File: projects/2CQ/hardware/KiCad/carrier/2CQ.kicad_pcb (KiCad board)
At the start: 2 copper layers, 48.5 x 111 mm, 17 parts, among them SW1 TOGGLE_ON-ON, U1 ES_DAISY_PATCH_SM_REV1

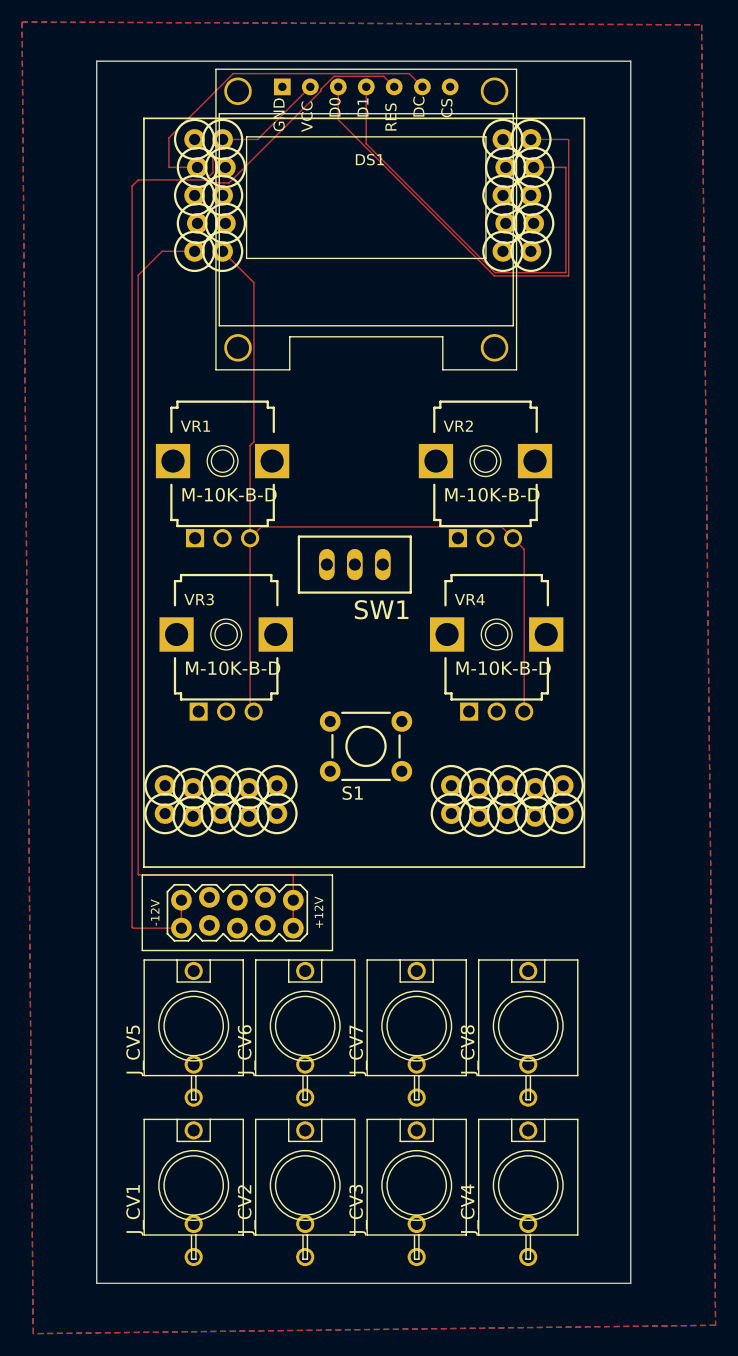
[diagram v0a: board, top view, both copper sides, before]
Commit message: routing organizing
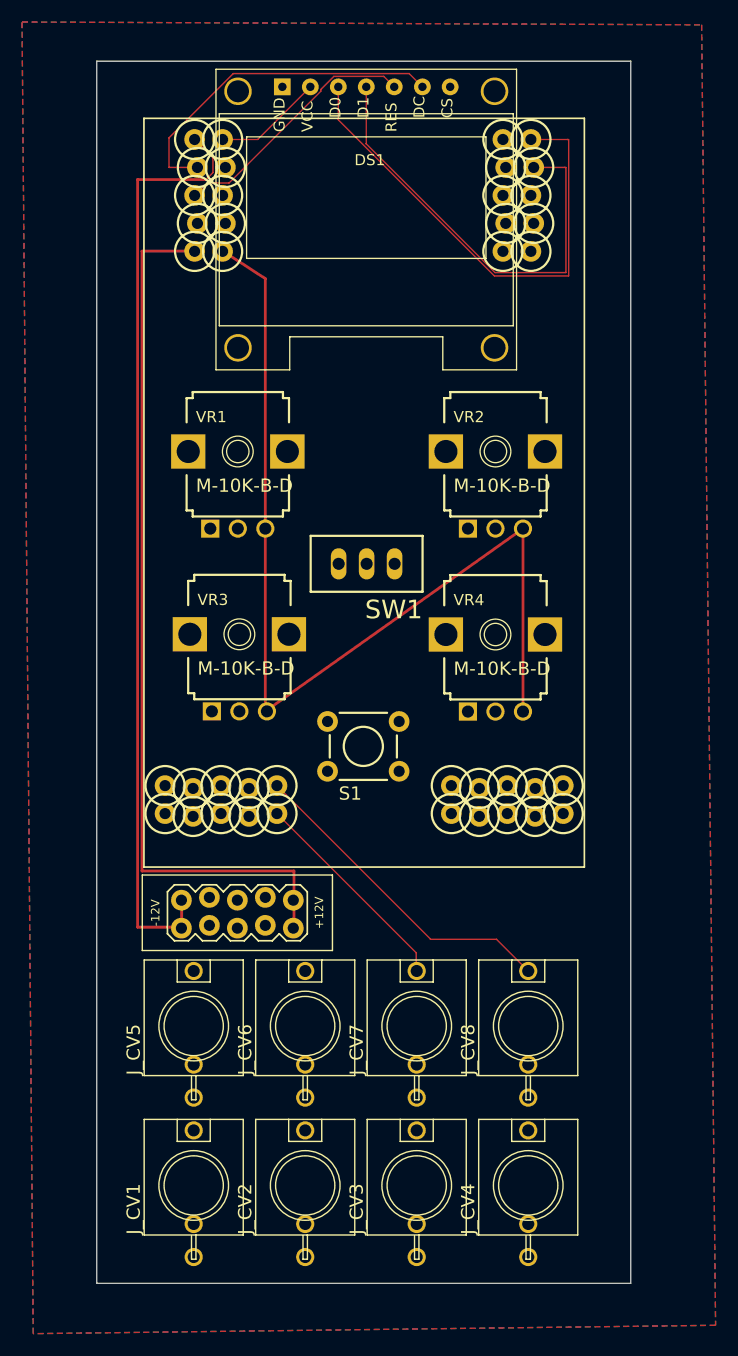
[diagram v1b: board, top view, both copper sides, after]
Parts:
- moved VR1 1.63 mm to (86.4, 79.9)
- moved VR2 1.26 mm to (109.8, 79.9)
- moved VR3 1.20 mm to (86.5, 96.5)
- moved SW1 1.07 mm to (98.1, 90.1)
- moved S1 0.24 mm to (97.8, 106.7)
- moved VR4 0.11 mm to (109.8, 96.5)
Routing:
- net +5V: track 84.1 -> 0.00 mm
- net -12V: track 85.9 -> 4.63 mm
- net +12V: track 79.5 -> 0.00 mm
- net /SIG_GATE_OUT_2: track 0.00 -> 29.8 mm
- net /SIG_GATE_OUT_1: track 0.00 -> 19.6 mm
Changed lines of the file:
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@@
 	(footprint "ES_Daisy_Patch_SM_FB_Rev1:TOGGLE_ON-ON"
 		(layer "F.Cu")
-		(at 97.028 90.17 180)
+		(at 98.1 90.1 180)
 		(property "Reference" "SW1"
 			(at -5.08 -3.175 0)
@@
 	(footprint "ES_Daisy_Patch_SM_FB_Rev1:9MM_SNAP-IN_POT_SILK"
 		(layer "F.Cu")
-		(at 85.344 96.52)
+		(at 86.544 96.50095)
 		(descr "9mm vertical snap-in pot, Alpha / Panasonic style")
 		(property "Reference" "VR3"
@@
 	(footprint "ES_Daisy_Patch_SM_FB_Rev1:TL1105SPF250Q_SILK"
 		(layer "F.Cu")
-		(at 98.044 106.68)
+		(at 97.8 106.68)
 		(property "Reference" "S1"
 			(at -2.24 4.99 180)
@@
 	(footprint "ES_Daisy_Patch_SM_FB_Rev1:9MM_SNAP-IN_POT_SILK"
 		(layer "F.Cu")
-		(at 85.018 80.772)
+		(at 86.4 79.9)
 		(descr "9mm vertical snap-in pot, Alpha / Panasonic style")
 		(property "Reference" "VR1"
@@
 	(footprint "ES_Daisy_Patch_SM_FB_Rev1:9MM_SNAP-IN_POT_SILK"
 		(layer "F.Cu")
-		(at 109.91 96.52)
+		(at 109.8 96.52)
 		(descr "9mm vertical snap-in pot, Alpha / Panasonic style")
 		(property "Reference" "VR4"
@@
 	(footprint "ES_Daisy_Patch_SM_FB_Rev1:9MM_SNAP-IN_POT_SILK"
 		(layer "F.Cu")
-		(at 108.894 80.772)
+		(at 109.8 79.9)
 		(descr "9mm vertical snap-in pot, Alpha / Panasonic style")
 		(property "Reference" "VR2"
@@
 	)
 	(gr_line
+		(start 88.9 86.7)
+		(end 88.9 64.2)
+		(stroke
+			(width 0.254)
+			(type default)
+		)
+		(layer "F.Cu")
+		(net 34)
+	)
+	(gr_line
+		(start 88.9 103.5)
+		(end 112.3 86.9)
+		(stroke
+			(width 0.254)
+			(type default)
+		)
+		(layer "F.Cu")
+		(net 34)
+	)
+	(gr_line
+		(start 112.3 86.9)
+		(end 112.3 103.5)
+		(stroke
+			(width 0.254)
+			(type default)
+		)
+		(layer "F.Cu")
+		(net 34)
+	)
+	(gr_line
+		(start 77.7 61.7)
+		(end 77.7 118)
+		(stroke
+			(width 0.254)
+			(type default)
+		)
+		(layer "F.Cu")
+		(net 8)
+	)
+	(gr_line
+		(start 77.7 118)
+		(end 91.5 118)
+		(stroke
+			(width 0.254)
+			(type default)
+		)
+		(layer "F.Cu")
+		(net 8)
+	)
+	(gr_line
+		(start 88.9 64.2)
+		(end 84.9 61.6)
+		(stroke
+			(width 0.254)
+			(type default)
+		)
+		(layer "F.Cu")
+		(net 34)
+	)
+	(gr_line
+		(start 77.3 123.1)
+		(end 81.3 123.1)
+		(stroke
+			(width 0.254)
+			(type default)
+		)
+		(layer "F.Cu")
+		(net 9)
+	)
+	(gr_line
+		(start 91.5 118)
+		(end 91.5 120.6)
+		(stroke
+			(width 0.254)
+			(type default)
+		)
+		(layer "F.Cu")
+		(net 8)
+	)
+	(gr_line
+		(start 81.3 123.1)
+		(end 81.3 120.7)
+		(stroke
+			(width 0.254)
+			(type default)
+		)
+		(layer "F.Cu")
+		(net 9)
+	)
+	(gr_line
+		(start 83.4 55.2)
+		(end 77.3 55.2)
+		(stroke
+			(width 0.254)
+			(type default)
+		)
+		(layer "F.Cu")
+		(net 9)
+	)
+	(gr_line
+		(start 91.5 120.6)
+		(end 91.5 123.2)
+		(stroke
+			(width 0.254)
+			(type default)
+		)
+		(layer "F.Cu")
+		(net 8)
+	)
+	(gr_line
+		(start 77.3 55.2)
+		(end 77.3 123.1)
+		(stroke
+			(width 0.254)
+			(type default)
+		)
+		(layer "F.Cu")
+		(net 9)
+	)
+	(gr_line
+		(start 88.9 86.7)
+		(end 88.9 103.5)
+		(stroke
+			(width 0.254)
+			(type default)
+		)
+		(layer "F.Cu")
+		(net 34)
+	)
+	(gr_line
+		(start 82.6 61.7)
+		(end 77.7 61.7)
+		(stroke
+			(width 0.254)
+			(type default)
+		)
+		(layer "F.Cu")
+		(net 8)
+	)
+	(gr_line
 		(start 73.914 118.872)
 		(end 73.914 125.73)
@@
 	)
 	(segment
-		(start 77.35 63.9)
-		(end 79.528 61.722)
-		(width 0.127)
-		(layer "F.Cu")
-		(net 8)
-	)
-	(segment
-		(start 79.528 61.722)
-		(end 82.478 61.722)
-		(width 0.127)
-		(layer "F.Cu")
-		(net 8)
-	)
-	(segment
-		(start 77.4 118.35)
-		(end 77.35 118.3)
-		(width 0.127)
-		(layer "F.Cu")
-		(net 8)
-	)
-	(segment
-		(start 77.35 118.3)
-		(end 77.35 63.9)
-		(width 0.127)
-		(layer "F.Cu")
-		(net 8)
-	)
-	(segment
-		(start 91.44 123.19)
-		(end 91.44 120.65)
-		(width 0.127)
-		(layer "F.Cu")
-		(net 8)
-	)
-	(segment
-		(start 91.44 120.65)
-		(end 91.44 118.41)
-		(width 0.127)
-		(layer "F.Cu")
-		(net 8)
-	)
-	(segment
-		(start 91.44 118.41)
-		(end 91.5 118.35)
-		(width 0.127)
-		(layer "F.Cu")
-		(net 8)
-	)
-	(segment
-		(start 91.5 118.35)
-		(end 77.4 118.35)
-		(width 0.127)
-		(layer "F.Cu")
-		(net 8)
-	)
-	(segment
-		(start 77.3667 55.2333)
-		(end 83.478 55.2333)
-		(width 0.127)
-		(layer "F.Cu")
-		(net 9)
-	)
-	(segment
-		(start 81.28 123.19)
-		(end 76.89 123.19)
-		(width 0.127)
-		(layer "F.Cu")
-		(net 9)
-	)
-	(segment
-		(start 81.28 120.65)
-		(end 81.28 123.19)
-		(width 0.127)
-		(layer "F.Cu")
-		(net 9)
-	)
-	(segment
-		(start 76.8 55.8)
-		(end 77.3667 55.2333)
-		(width 0.127)
-		(layer "F.Cu")
-		(net 9)
-	)
-	(segment
-		(start 76.89 123.19)
-		(end 76.8 123.1)
-		(width 0.127)
-		(layer "F.Cu")
-		(net 9)
-	)
-	(segment
 		(start 84.1407 54.5706)
 		(end 84.1407 53.2247)
@@
 	)
 	(segment
-		(start 76.8 123.1)
-		(end 76.8 55.8)
-		(width 0.127)
-		(layer "F.Cu")
-		(net 9)
-	)
-	(segment
 		(start 83.478 55.2333)
 		(end 84.1407 54.5706)
@@
 	)
 	(segment
-		(start 87.518 79.363)
-		(end 87.518 87.772)
-		(width 0.127)
-		(layer "F.Cu")
-		(net 34)
-	)
-	(segment
-		(start 87.8585 79.0225)
-		(end 87.518 79.363)
-		(width 0.127)
-		(layer "F.Cu")
-		(net 34)
-	)
-	(segment
-		(start 87.518 87.772)
-		(end 87.518 103.194)
-		(width 0.127)
-		(layer "F.Cu")
-		(net 34)
-	)
-	(segment
-		(start 87.518 103.194)
-		(end 87.844 103.52)
+		(start 102.6 127.031)
+		(end 102.649 127.08)
 		(width 0.127)
 		(layer "F.Cu")
-		(net 34)
-	)
-	(segment
-		(start 87.518 87.772)
-		(end 88.5345 86.7555)
-		(width 0.127)
-		(layer "F.Cu")
-		(net 34)
+		(net 25)
 	)
 	(segment
-		(start 112.41 88.788)
-		(end 112.41 103.52)
+		(start 89.955 112.785)
+		(end 102.6 125.43)
 		(width 0.127)
 		(layer "F.Cu")
-		(net 34)
+		(net 25)
 	)
 	(segment
-		(start 111.394 87.772)
-		(end 112.41 88.788)
+		(start 102.6 125.43)
+		(end 102.6 127.031)
 		(width 0.127)
 		(layer "F.Cu")
-		(net 34)
+		(net 25)
 	)
 	(segment
-		(start 88.5345 86.7555)
-		(end 110.3775 86.7555)
+		(start 103.9 124.19)
+		(end 103.9 124.2)
 		(width 0.127)
 		(layer "F.Cu")
-		(net 34)
+		(net 26)
 	)
 	(segment
-		(start 110.3775 86.7555)
-		(end 111.394 87.772)
+		(start 103.9 124.2)
+		(end 109.896 124.2)
 		(width 0.127)
 		(layer "F.Cu")
-		(net 34)
+		(net 26)
 	)
 	(segment
-		(start 85.018 61.722)
-		(end 87.8585 64.5625)
+		(start 109.896 124.2)
+		(end 112.776 127.08)
 		(width 0.127)
 		(layer "F.Cu")
-		(net 34)
+		(net 26)
 	)
 	(segment
-		(start 87.8585 64.5625)
-		(end 87.8585 79.0225)
+		(start 89.955 110.245)
+		(end 103.9 124.19)
 		(width 0.127)
 		(layer "F.Cu")
-		(net 34)
+		(net 26)
 	)
 	(zone
